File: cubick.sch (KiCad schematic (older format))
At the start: 8 parts

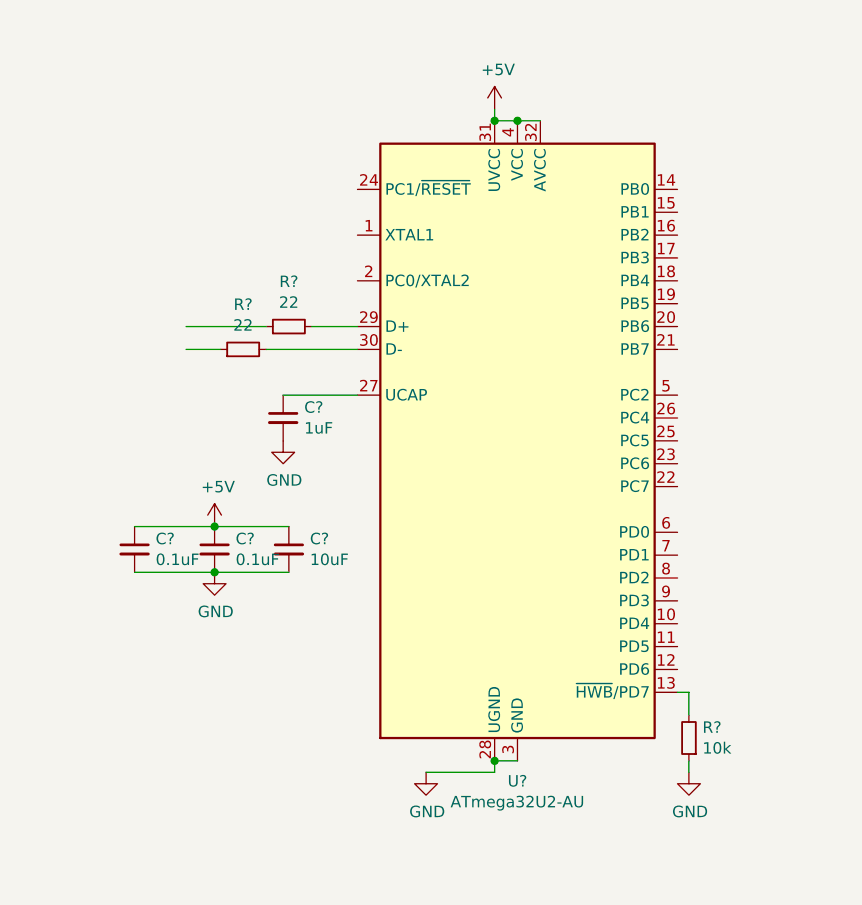
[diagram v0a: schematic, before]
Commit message: 2019-11-14 32u2 susunda
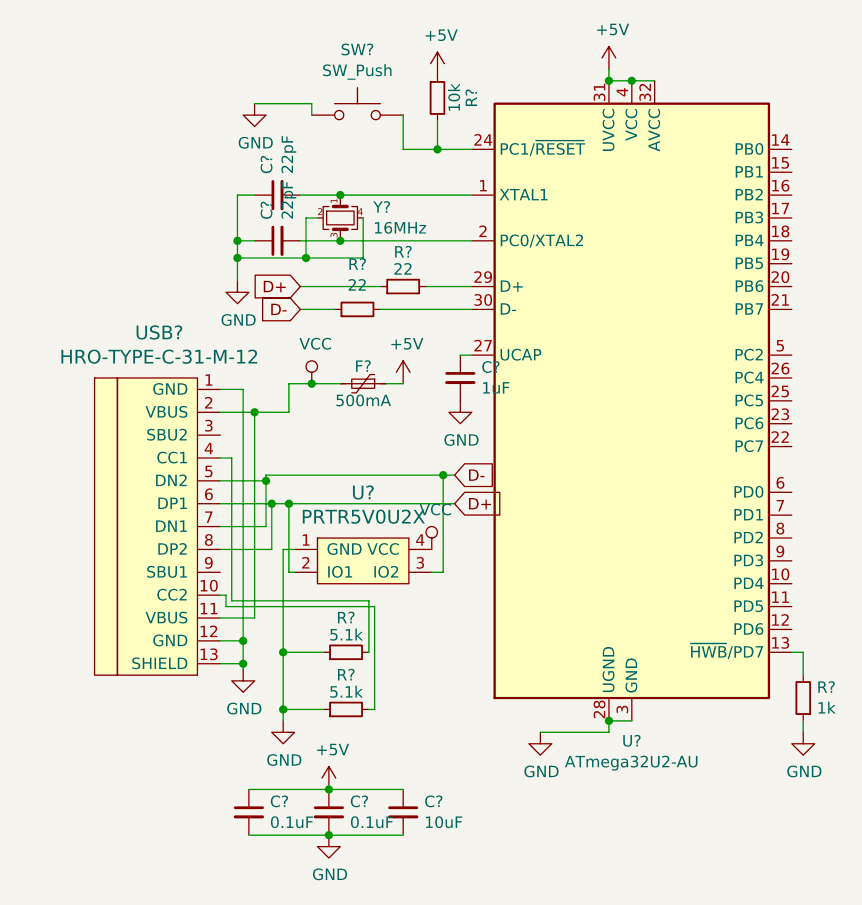
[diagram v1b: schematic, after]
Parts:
- added C? (x2): 22pF, symbol Device:C_Small
- added F?: 500mA, symbol Device:Polyfuse_Small
- added R?: 10k, symbol Device:R_Small
- added R? (x2): 5.1k, symbol Device:R_Small
- added SW?: SW_Push, symbol Switch:SW_Push
- added U?: PRTR5V0U2X, symbol random-keyboard-parts:PRTR5V0U2X
- added USB?: HRO-TYPE-C-31-M-12, symbol Type-C:HRO-TYPE-C-31-M-12
- added Y?: 16MHz, symbol Device:Crystal_GND24_Small
- R?: value 10k -> 1k
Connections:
- net labels added: D+, D-, VCC
- wire segments 18 -> 82
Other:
- moved on the sheet: C?, R?, U?
